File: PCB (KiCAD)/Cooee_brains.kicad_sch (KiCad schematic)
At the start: 29 parts, among them J1 USB4105-GF-A, J4 Conn_01x14_Socket, J5 Conn_02x20_Counter_Clockwise, SW1 Prog, SW2 Reset, U1 AMS1117-3.3, U2 ESP32-S3-WROOM-1-N8, U3 SX1262IMLTRT, U4 RXM-GPS-FM

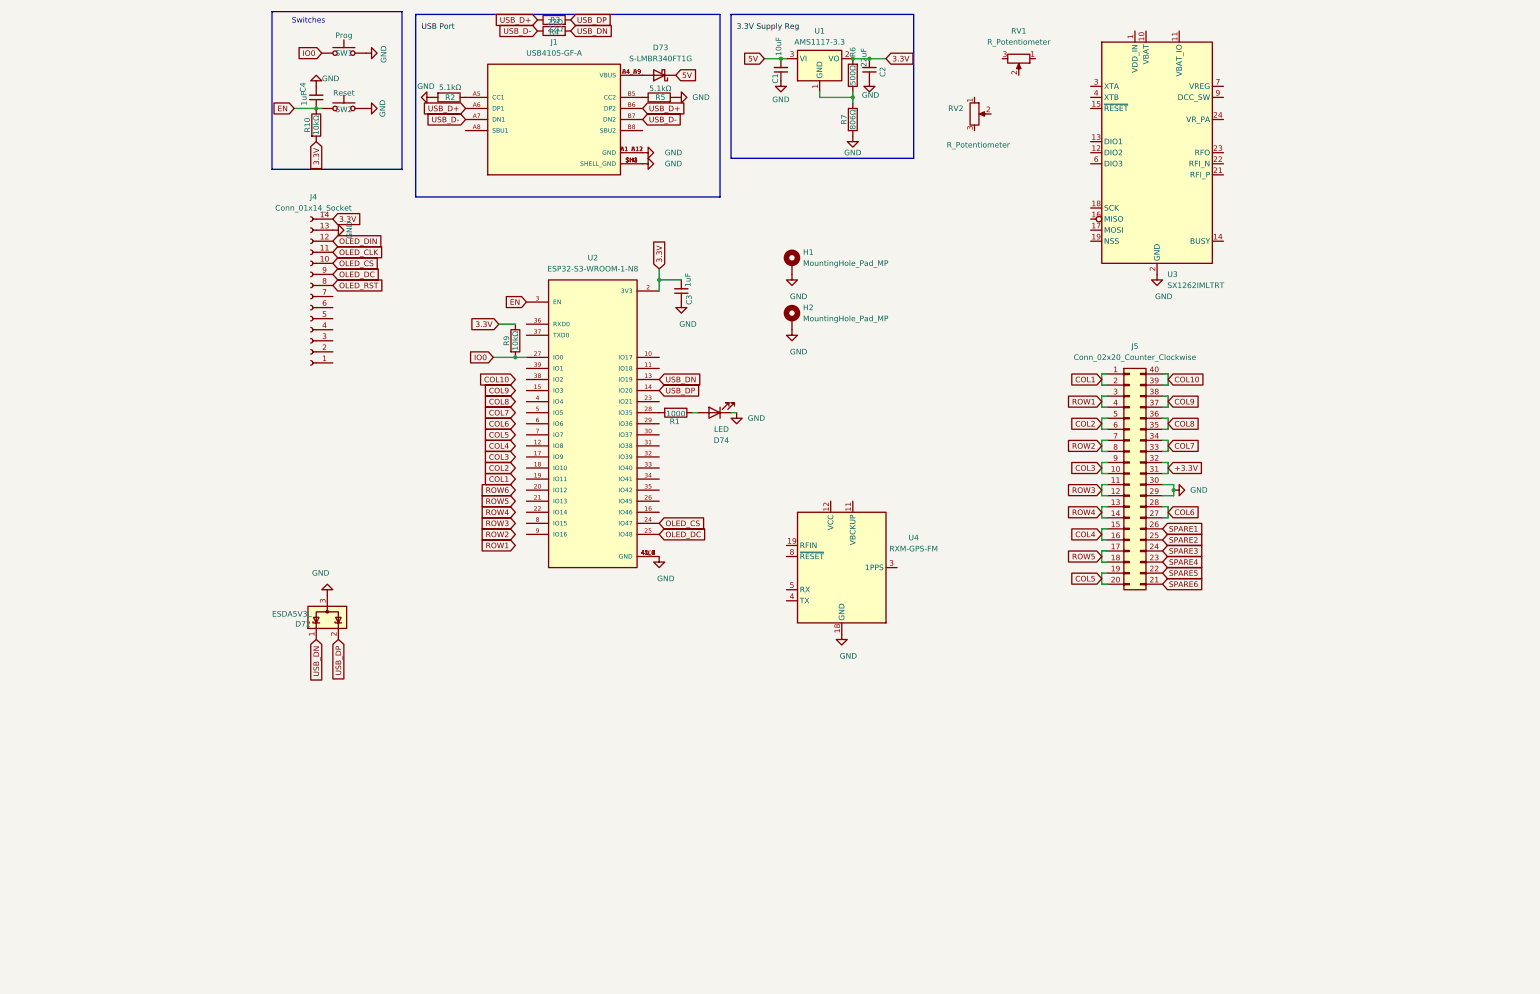
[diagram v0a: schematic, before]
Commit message: motherboard PCB layout work
motherboard PCB layout work
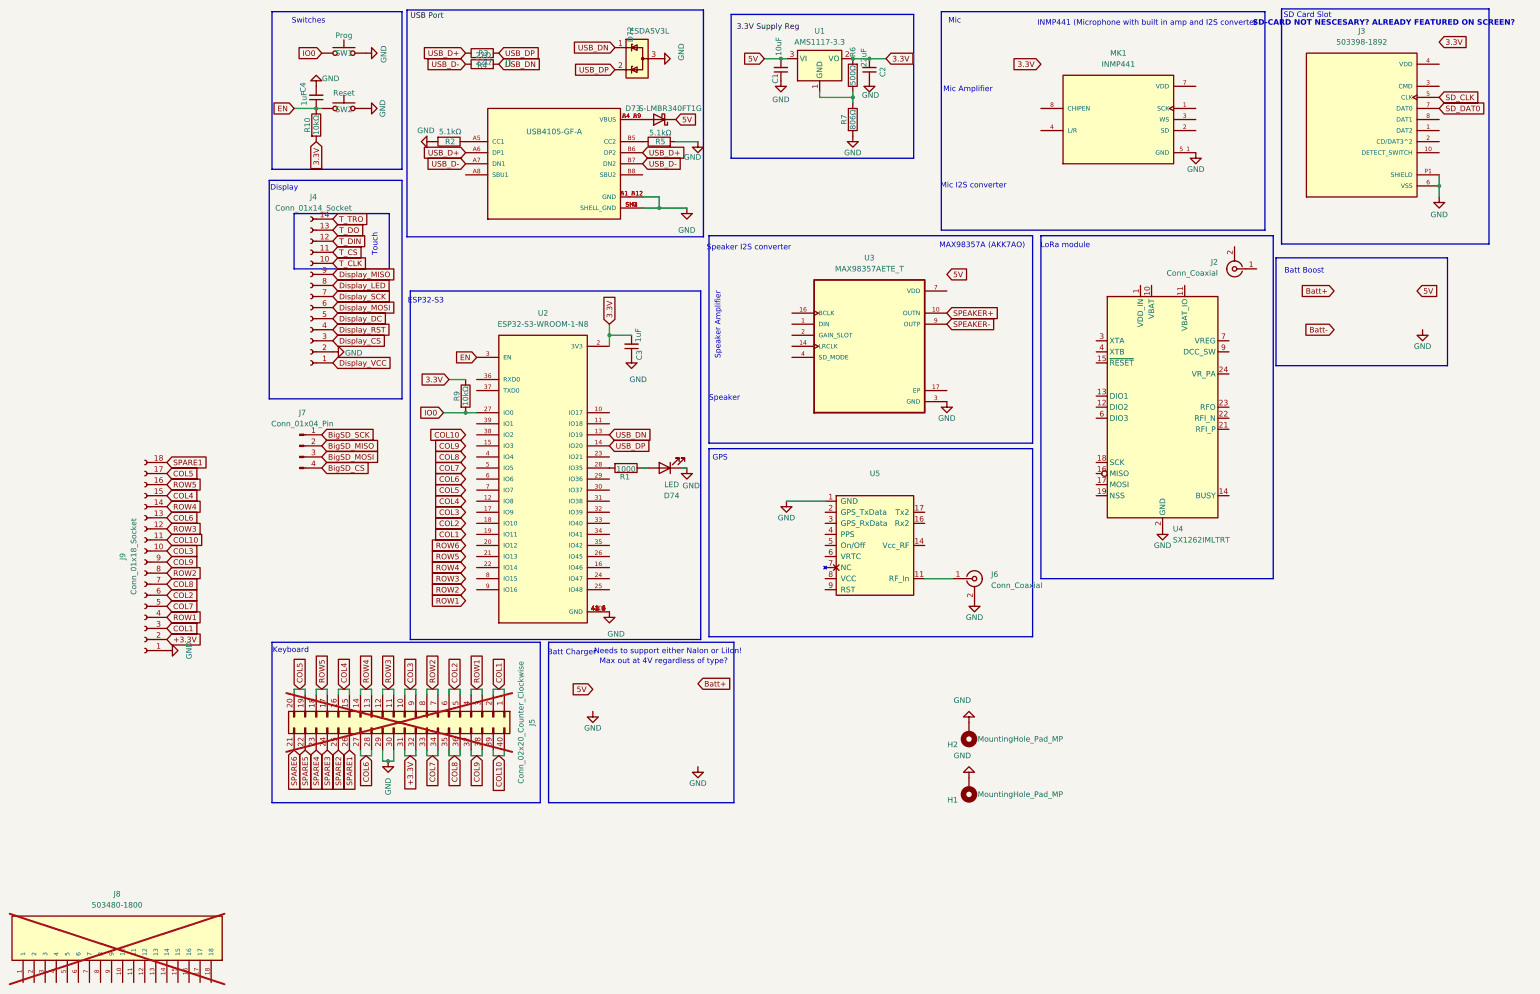
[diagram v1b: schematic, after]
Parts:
- removed RV1, RV2: R_Potentiometer, symbol Device:R_Potentiometer
- removed U3: SX1262IMLTRT, Package_DFN_QFN:QFN-24-1EP_4x4mm_P0.5mm_EP2.6x2.6mm, symbol RF:SX1262IMLTRT
- removed U4: RXM-GPS-FM, RF_GPS:Linx_RXM-GPS, symbol RF_GPS:RXM-GPS-FM
- added J2, J6: Conn_Coaxial, Connector_Coaxial:U.FL_Molex_MCRF_73412-0110_Vertical, symbol Connector:Conn_Coaxial
- added J3: 503398-1892, USB4105-GF-A (1):MOLEX_503398-1892, symbol Downloaded:503398-1892
- added J7: Conn_01x04_Pin, Connector_PinHeader_2.54mm:PinHeader_1x04_P2.54mm_Horizontal, symbol Connector:Conn_01x04_Pin
- added J8: 503480-1800, USB4105-GF-A (1):MOLEX_503480-1800, symbol Downloaded:503480-1800
- added J9: Conn_01x18_Socket, Connector_PinSocket_2.54mm:PinSocket_1x18_P2.54mm_Vertical_SMD_Pin1Left, symbol Connector:Conn_01x18_Socket
- added MK1: INMP441, USB4105-GF-A (1):MIC_INMP441, symbol Downloaded:INMP441
- added U3: MAX98357AETE_T, MAX98357AETE_T:QFN50P300X300X80-17N, symbol Downloaded:MAX98357AETE_T
- added U4: SX1262IMLTRT, Package_DFN_QFN:QFN-24-1EP_4x4mm_P0.5mm_EP2.6x2.6mm, symbol RF:SX1262IMLTRT
- added U5: ~, USB4105-GF-A (1):M210Z, symbol Downloaded:M210Z
- J4: footprint Connector_PinSocket_2.54mm:PinSocket_1x14_P2.54mm_Vertical -> Connector_PinSocket_2.54mm:PinSocket_1x14_P2.54mm_Horizontal
- J5: now not fitted; now left out of the parts list
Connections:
- net +3.3V: now also J9.2 (Pin_2)
- net 3.3V: no longer J4.14 (Pin_14)
- net COL1: now also J9.3 (Pin_3)
- net COL10: now also J9.11 (Pin_11)
- net COL2: now also J9.6 (Pin_6)
- net COL3: now also J9.10 (Pin_10)
- net COL4: now also J9.15 (Pin_15)
- net COL5: now also J9.17 (Pin_17)
- net COL6: now also J9.13 (Pin_13)
- net COL7: now also J9.5 (Pin_5)
- net COL8: now also J9.7 (Pin_7)
- net COL9: now also J9.9 (Pin_9)
- net GND: now also J4.2 (Pin_2), J3.6 (VSS), J3.9 (VSS), J3.P1 (SHIELD), J3.P2 (SHIELD), J3.P3 (SHIELD), J3.P4 (SHIELD), J6.2 (Ext), J9.1 (Pin_1), MK1.5_1 (GND), MK1.5_2 (GND), MK1.6 (GND), MK1.9 (GND), U3.11 (GND), U3.15 (GND), U3.3 (GND), U4.2 (GND), U4.20 (GND), U4.25 (GND), U4.5 (GND), U4.8 (GND), U5.1 (GND); no longer J4.13 (Pin_13)
- net ROW1: now also J9.4 (Pin_4)
- net ROW2: now also J9.8 (Pin_8)
- net ROW3: now also J9.12 (Pin_12)
- net ROW4: now also J9.14 (Pin_14)
- net ROW5: now also J9.16 (Pin_16)
- net SPARE1: now also J9.18 (Pin_18)
- net Display_VCC: now reaches J4.1 (Pin_1)
- net Display_CS: now reaches J4.3 (Pin_3)
- net Display_RST: now reaches J4.4 (Pin_4)
- net Display_DC: now reaches J4.5 (Pin_5)
- net Display_MOSI: now reaches J4.6 (Pin_6)
- net Display_SCK: now reaches J4.7 (Pin_7)
- net OLED_CLK renamed T_CS
- net OLED_CS: no longer names the net of U2.24 (IO47)
- net OLED_CS: no longer J4.10 (Pin_10)
- net OLED_DC: no longer names the net of U2.25 (IO48)
- net OLED_DC: no longer J4.9 (Pin_9)
- net OLED_DIN renamed T_DIN
- net OLED_RST renamed Display_LED
- new net: J6.1 (In), U5.11 (RF_In)
- new net BigSD_CS: J7.4 (Pin_4)
- new net BigSD_MISO: J7.2 (Pin_2)
- new net BigSD_MOSI: J7.3 (Pin_3)
- new net BigSD_SCK: J7.1 (Pin_1)
- new net Display_MISO: J4.9 (Pin_9)
- new net SD_CLK: J3.5 (CLK)
- new net SD_DAT0: J3.7 (DAT0)
- new net SPEAKER+: U3.10 (OUTN)
- new net SPEAKER-: U3.9 (OUTP)
- new net T_CLK: J4.10 (Pin_10)
- new net T_DO: J4.13 (Pin_13)
- new net T_TRO: J4.14 (Pin_14)
- new net VDD: U3.7 (VDD), U3.8 (VDD)
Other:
- note added: "(AKK7AO)"
- note added: "Batt Boost"
- note added: "Batt Charger"
- note added: "Display"
- note added: "ESP32-S3"
- note added: "GPS"
- note added: "INMP441 (Microphone with built in amp and I2S converter"
- note added: "Keyboard"
- note added: "LoRa module"
- note added: "MAX98357A"
- note added: "Max out at 4V regardless of type?"
- note added: "Mic"
- note added: "Mic Amplifier"
- note added: "Mic I2S converter"
- note added: "Needs to support either NaIon or LiIon!"
- note added: "SD Card Slot"
- note added: "SD-CARD NOT NESCESARY? ALREADY FEATURED ON SCREEN?"
- note added: "Speaker"
- note added: "Speaker Amplifier"
- note added: "Speaker I2S converter"
- note added: "Touch"
- moved on the sheet: C3, D72, D73, D74, H1, H2, J1, R1, R2, R3, R4, R5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
